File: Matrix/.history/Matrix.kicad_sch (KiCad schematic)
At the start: 55 parts, among them J1 Conn_01x08, Q1 2N2219, Q10 2N2219, Q11 2N2219, Q12 2N2219, Q13 2N2219, Q14 2N2219, Q15 2N2219, Q16 2N2219, Q2 2N2219, Q3 2N2219, Q4 2N2219, Q5 2N2219, Q6 2N2219, Q7 2N2219, Q8 2N2219, Q9 2N2219, U1 74HC138

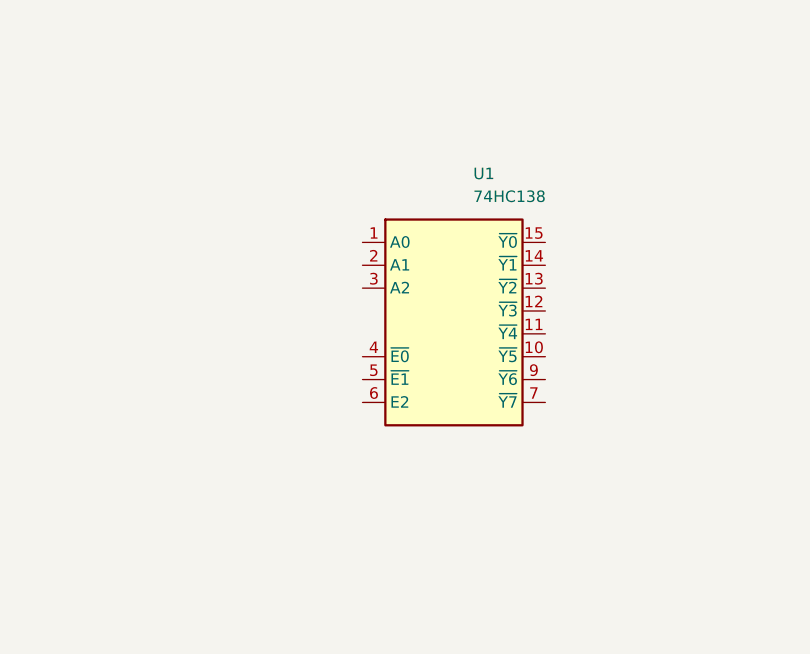
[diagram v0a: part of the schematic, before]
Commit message: Update Matrix.kicad_sch
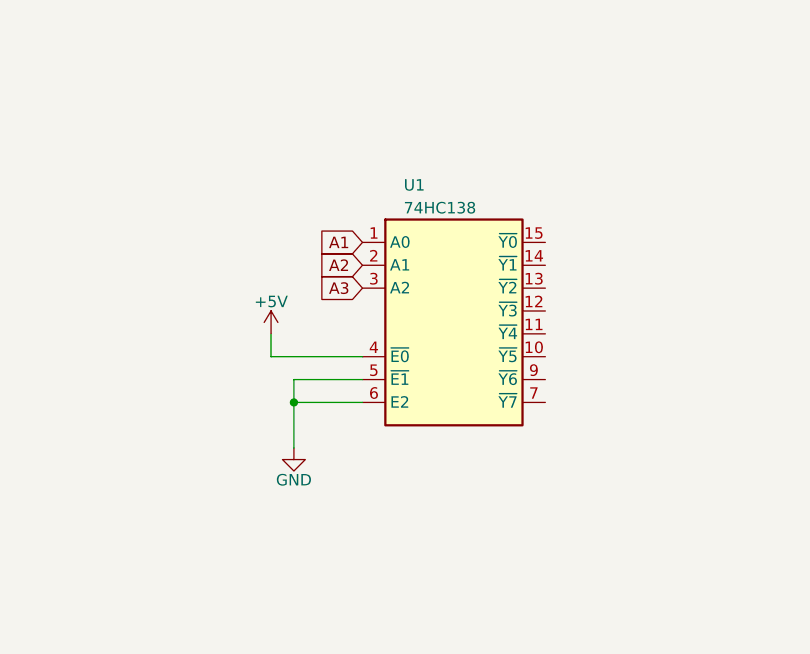
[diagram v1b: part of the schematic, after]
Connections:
- net +5V: now also U1.4 (~{E0})
- net A1: now also U1.1 (A0)
- net A2: now also U1.2 (A1)
- net A3: now also U1.3 (A2)
- net GND: now also U1.5 (~{E1}), U1.6 (E2)
